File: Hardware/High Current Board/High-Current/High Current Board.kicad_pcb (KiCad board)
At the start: 2 copper layers, 174.9 x 151.1 mm, 37 parts, among them J1 8P8C_Shielded, J2 Conn_01x04, J3 GND, J4 Load Resistors Return, J5 +46V from Fuel Cell, K1 G2RL-1A-E, K2 G2RL-1A-E, Q1 NMOS_Substrate, U1 TC4421AVAT, U3 HO 25-P

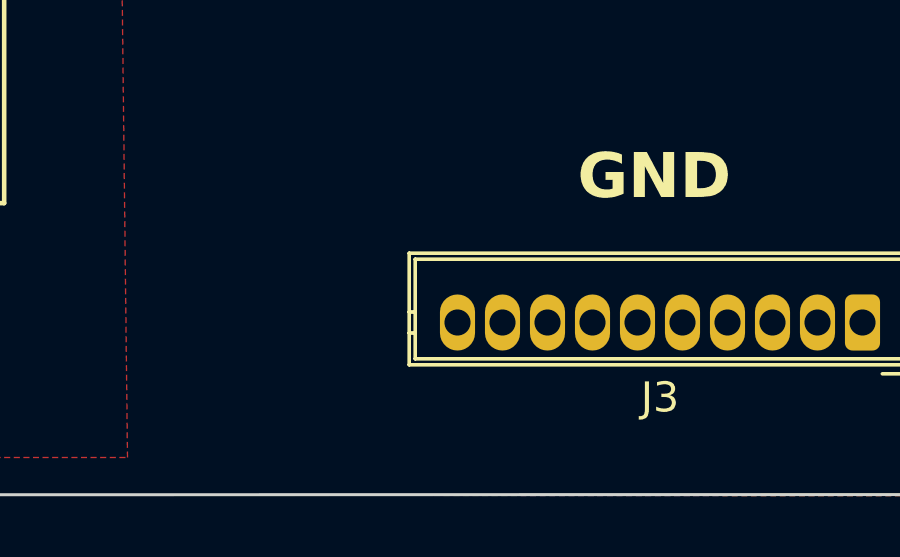
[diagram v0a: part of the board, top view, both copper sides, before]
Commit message: Text update
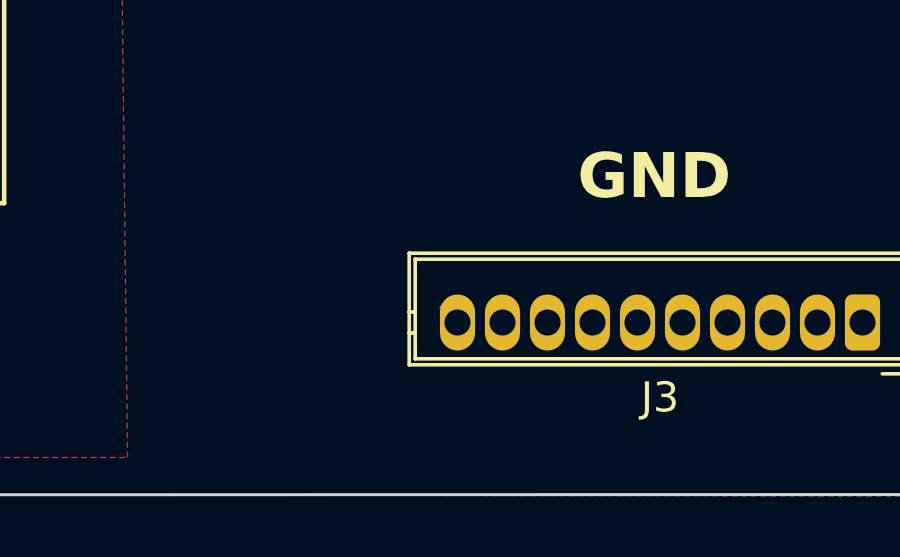
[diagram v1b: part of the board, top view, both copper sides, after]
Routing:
- net (no net): track 0.00 -> 0.71 mm
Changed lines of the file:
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@@
     (date "2024-01-11")
     (rev "0.0")
-    (comment 1 "University of Alberta EcoCar Team")
-    (comment 2 "Automated Resistive Load Bank Project")
+    (company "University of Alberta EcoCar Team")
+    (comment 1 "Automated Resistive Load Bank Project")
+    (comment 6 " ")
   )
   (layers
@@
     (effects (font (size 1.5 1.5) (thickness 0.3) bold) (justify left bottom))
   )
+  (segment (start 196 159.25) (end 195.5 158.75) (width 0.2) (layer "B.Cu") (net 0))
   (segment (start 149.116 154.25) (end 149.066 154.2) (width 0.2) (layer "F.Cu") (net 1))
   (segment (start 139.85 155.6) (end 139 154.75) (width 0.2) (layer "F.Cu") (net 1))
